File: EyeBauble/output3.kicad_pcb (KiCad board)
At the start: 2 copper layers, 8.6 x 31.9 mm, 48 parts

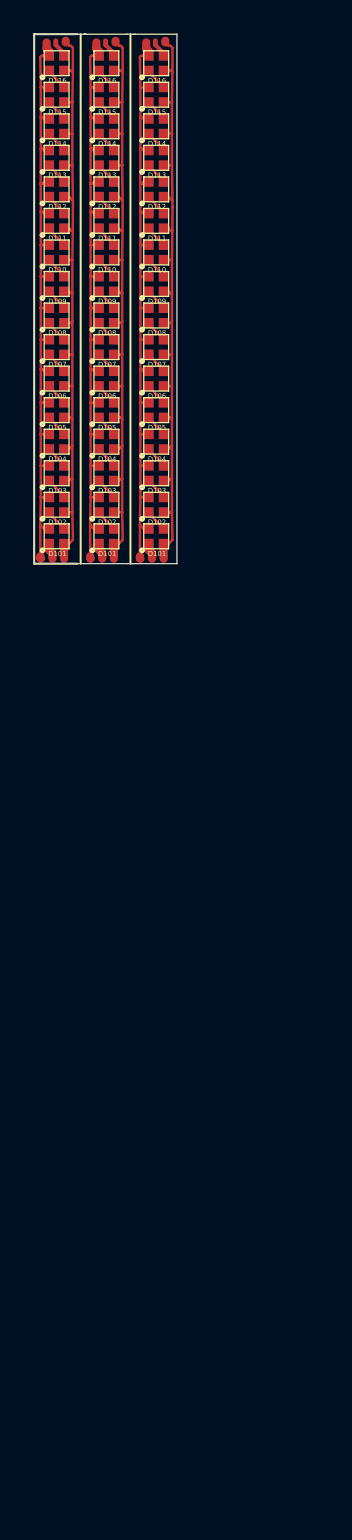
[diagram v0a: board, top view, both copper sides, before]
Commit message: Dunno what I'm committing but this was the latest rev
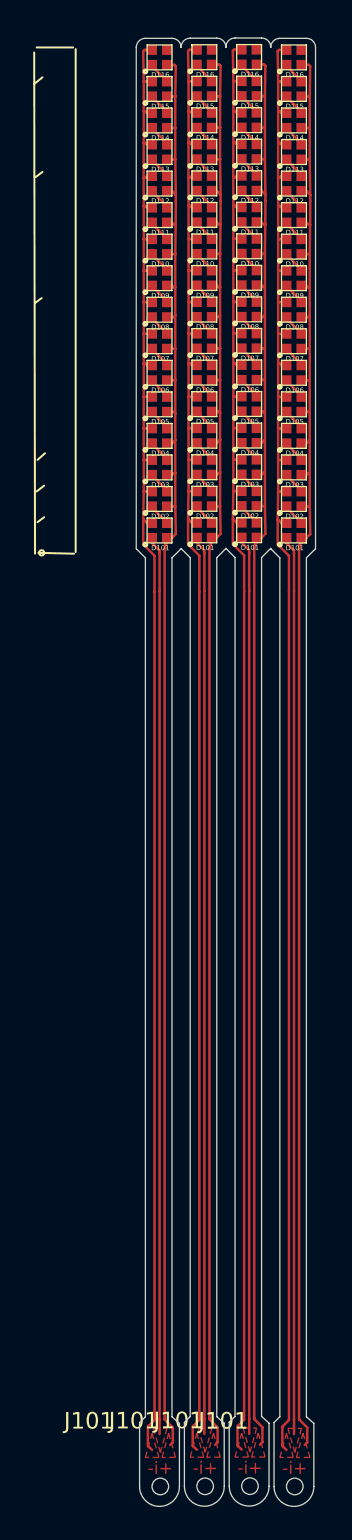
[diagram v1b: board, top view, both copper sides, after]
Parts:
- removed the D101 at (86.4, 75.0)
- removed the D101 at (83.4, 75.0)
- removed the D102 at (86.4, 73.1)
- removed the D102 at (83.4, 73.1)
- removed the D103 at (86.4, 71.2)
- removed the D103 at (83.4, 71.2)
- removed the D104 at (86.4, 69.3)
- removed the D104 at (83.4, 69.3)
- removed the D105 at (86.4, 67.4)
- removed the D105 at (83.4, 67.4)
- removed the D106 at (86.4, 65.5)
- removed the D106 at (83.4, 65.5)
- removed the D107 at (86.4, 63.6)
- removed the D107 at (83.4, 63.6)
- removed the D108 at (86.4, 61.7)
- removed the D108 at (83.4, 61.7)
- removed the D109 at (86.4, 59.8)
- removed the D109 at (83.4, 59.8)
- removed the D110 at (86.4, 57.9)
- removed the D110 at (83.4, 57.9)
- removed the D111 at (86.4, 56.0)
- removed the D111 at (83.4, 56.0)
- removed the D112 at (86.4, 54.1)
- removed the D112 at (83.4, 54.1)
- removed the D113 at (86.4, 52.2)
- removed the D113 at (83.4, 52.2)
- removed the D114 at (86.4, 50.3)
- removed the D114 at (83.4, 50.3)
- removed the D115 at (86.4, 48.4)
- removed the D115 at (83.4, 48.4)
- removed the D116 at (86.4, 46.5)
- removed the D116 at (83.4, 46.5)
- added D101: SK6812MINI, SK6812-EC1515:SK6812-EC1515, F.Cu at (94.7, 74.6)
- added D101: SK6812MINI, SK6812-EC1515:SK6812-EC1515, F.Cu at (92.0, 74.6)
- added D101: SK6812MINI, SK6812-EC1515:SK6812-EC1515, F.Cu at (89.3, 74.6)
- added D102: SK6812MINI, SK6812-EC1515:SK6812-EC1515, F.Cu at (94.7, 72.7)
- added D102: SK6812MINI, SK6812-EC1515:SK6812-EC1515, F.Cu at (92.0, 72.7)
- added D102: SK6812MINI, SK6812-EC1515:SK6812-EC1515, F.Cu at (89.3, 72.7)
- added D103: SK6812MINI, SK6812-EC1515:SK6812-EC1515, F.Cu at (94.7, 70.8)
- added D103: SK6812MINI, SK6812-EC1515:SK6812-EC1515, F.Cu at (92.0, 70.8)
- added D103: SK6812MINI, SK6812-EC1515:SK6812-EC1515, F.Cu at (89.3, 70.8)
- added D104: SK6812MINI, SK6812-EC1515:SK6812-EC1515, F.Cu at (94.7, 68.9)
- added D104: SK6812MINI, SK6812-EC1515:SK6812-EC1515, F.Cu at (92.0, 68.9)
- added D104: SK6812MINI, SK6812-EC1515:SK6812-EC1515, F.Cu at (89.3, 68.9)
- added D105: SK6812MINI, SK6812-EC1515:SK6812-EC1515, F.Cu at (94.7, 67.0)
- added D105: SK6812MINI, SK6812-EC1515:SK6812-EC1515, F.Cu at (92.0, 67.0)
- added D105: SK6812MINI, SK6812-EC1515:SK6812-EC1515, F.Cu at (89.3, 67.0)
- added D106: SK6812MINI, SK6812-EC1515:SK6812-EC1515, F.Cu at (94.7, 65.1)
- added D106: SK6812MINI, SK6812-EC1515:SK6812-EC1515, F.Cu at (92.0, 65.1)
- added D106: SK6812MINI, SK6812-EC1515:SK6812-EC1515, F.Cu at (89.3, 65.1)
- added D107: SK6812MINI, SK6812-EC1515:SK6812-EC1515, F.Cu at (94.7, 63.2)
- added D107: SK6812MINI, SK6812-EC1515:SK6812-EC1515, F.Cu at (92.0, 63.2)
- added D107: SK6812MINI, SK6812-EC1515:SK6812-EC1515, F.Cu at (89.3, 63.2)
- added D108: SK6812MINI, SK6812-EC1515:SK6812-EC1515, F.Cu at (94.7, 61.3)
- added D108: SK6812MINI, SK6812-EC1515:SK6812-EC1515, F.Cu at (92.0, 61.3)
- added D108: SK6812MINI, SK6812-EC1515:SK6812-EC1515, F.Cu at (89.3, 61.3)
- added D109: SK6812MINI, SK6812-EC1515:SK6812-EC1515, F.Cu at (94.7, 59.4)
- added D109: SK6812MINI, SK6812-EC1515:SK6812-EC1515, F.Cu at (92.0, 59.4)
- added D109: SK6812MINI, SK6812-EC1515:SK6812-EC1515, F.Cu at (89.3, 59.4)
- added D110: SK6812MINI, SK6812-EC1515:SK6812-EC1515, F.Cu at (94.7, 57.5)
- added D110: SK6812MINI, SK6812-EC1515:SK6812-EC1515, F.Cu at (92.0, 57.5)
- added D110: SK6812MINI, SK6812-EC1515:SK6812-EC1515, F.Cu at (89.3, 57.5)
- added D111: SK6812MINI, SK6812-EC1515:SK6812-EC1515, F.Cu at (94.7, 55.6)
- added D111: SK6812MINI, SK6812-EC1515:SK6812-EC1515, F.Cu at (92.0, 55.6)
- added D111: SK6812MINI, SK6812-EC1515:SK6812-EC1515, F.Cu at (89.3, 55.6)
- added D112: SK6812MINI, SK6812-EC1515:SK6812-EC1515, F.Cu at (94.7, 53.7)
- added D112: SK6812MINI, SK6812-EC1515:SK6812-EC1515, F.Cu at (92.0, 53.7)
- added D112: SK6812MINI, SK6812-EC1515:SK6812-EC1515, F.Cu at (89.3, 53.7)
- added D113: SK6812MINI, SK6812-EC1515:SK6812-EC1515, F.Cu at (94.7, 51.8)
- added D113: SK6812MINI, SK6812-EC1515:SK6812-EC1515, F.Cu at (92.0, 51.8)
- added D113: SK6812MINI, SK6812-EC1515:SK6812-EC1515, F.Cu at (89.3, 51.8)
- added D114: SK6812MINI, SK6812-EC1515:SK6812-EC1515, F.Cu at (94.7, 49.9)
- added D114: SK6812MINI, SK6812-EC1515:SK6812-EC1515, F.Cu at (92.0, 49.9)
- added D114: SK6812MINI, SK6812-EC1515:SK6812-EC1515, F.Cu at (89.3, 49.9)
- added D115: SK6812MINI, SK6812-EC1515:SK6812-EC1515, F.Cu at (94.7, 48.0)
- added D115: SK6812MINI, SK6812-EC1515:SK6812-EC1515, F.Cu at (92.0, 48.0)
- added D115: SK6812MINI, SK6812-EC1515:SK6812-EC1515, F.Cu at (89.3, 48.0)
- added D116: SK6812MINI, SK6812-EC1515:SK6812-EC1515, F.Cu at (94.7, 46.1)
- added D116: SK6812MINI, SK6812-EC1515:SK6812-EC1515, F.Cu at (92.0, 46.1)
- added D116: SK6812MINI, SK6812-EC1515:SK6812-EC1515, F.Cu at (89.3, 46.1)
- added J101: Conn_01x01_Female, MountingHole:MountingHole_2.5mm, F.Cu at (95.2, 131.8)
- added J101: Conn_01x01_Female, MountingHole:MountingHole_2.5mm, F.Cu at (92.5, 131.8)
- added J101: Conn_01x01_Female, MountingHole:MountingHole_2.5mm, F.Cu at (89.8, 131.8)
- added J101: Conn_01x01_Female, MountingHole:MountingHole_2.5mm, F.Cu at (87.1, 131.8)
- moved D101 6.21 mm to (86.6, 74.6)
- moved D102 6.21 mm to (86.6, 72.7)
- moved D103 6.21 mm to (86.6, 70.8)
- moved D104 6.21 mm to (86.6, 68.9)
- moved D105 6.21 mm to (86.6, 67.0)
- moved D106 6.21 mm to (86.6, 65.1)
- moved D107 6.21 mm to (86.6, 63.2)
- moved D108 6.21 mm to (86.6, 61.3)
- moved D109 6.21 mm to (86.6, 59.4)
- moved D110 6.21 mm to (86.6, 57.5)
- moved D111 6.21 mm to (86.6, 55.6)
- moved D112 6.21 mm to (86.6, 53.7)
- moved D113 6.21 mm to (86.6, 51.8)
- moved D114 6.21 mm to (86.6, 49.9)
- moved D115 6.21 mm to (86.6, 48.0)
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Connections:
- D101 pad 1: (no net) -> /INPUT
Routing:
- net GND: track 118.5 -> 372.9 mm
- net +5V: track 119.6 -> 367.3 mm
- net /INPUT: track 0.00 -> 216.7 mm
- net (no net): track 6.26 -> 0.00 mm
- net Net-(D101-Pad3): track 4.13 -> 5.51 mm
- net Net-(D102-Pad3): track 4.13 -> 5.51 mm
- net Net-(D103-Pad3): track 4.13 -> 5.50 mm
- net Net-(D104-Pad3): track 4.13 -> 5.50 mm
- net Net-(D105-Pad3): track 4.13 -> 5.50 mm
- net Net-(D106-Pad3): track 4.13 -> 5.50 mm
- net Net-(D107-Pad3): track 4.13 -> 5.50 mm
- net Net-(D108-Pad3): track 4.12 -> 5.50 mm
- net Net-(D109-Pad3): track 4.12 -> 5.50 mm
- net Net-(D110-Pad3): track 4.12 -> 5.50 mm
- net Net-(D111-Pad3): track 4.12 -> 5.50 mm
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- added copper zone on F.Cu, net +5V
- added copper zone on F.Cu, net /INPUT
- added copper zone on F.Cu, net GND
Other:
- board size 8.6 x 31.9 mm -> 10.8 x 88.5 mm
- rule trace_min: 0.1524 -> 0.06
- board text added: "-i+"
